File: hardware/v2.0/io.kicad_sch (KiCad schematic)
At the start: 1 part, among them U1 ECP5U-25F-CABGA256

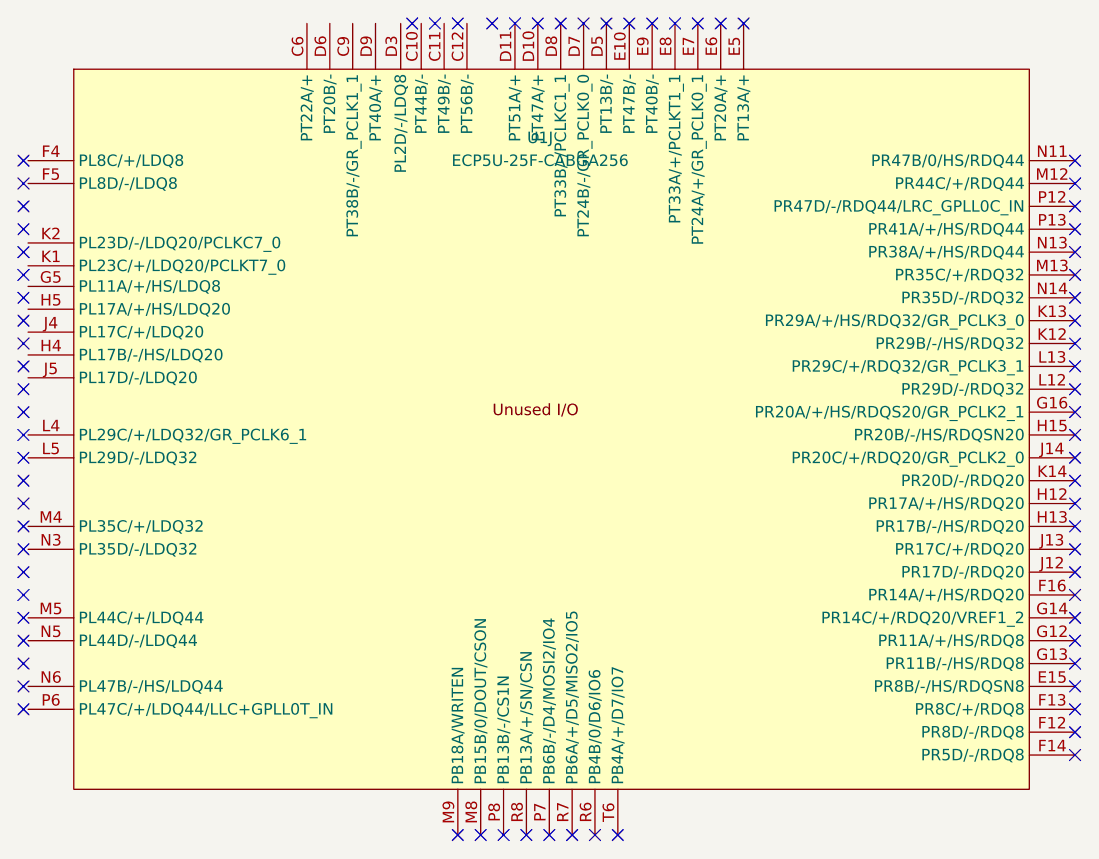
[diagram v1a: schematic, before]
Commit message: ADC SPI SDO
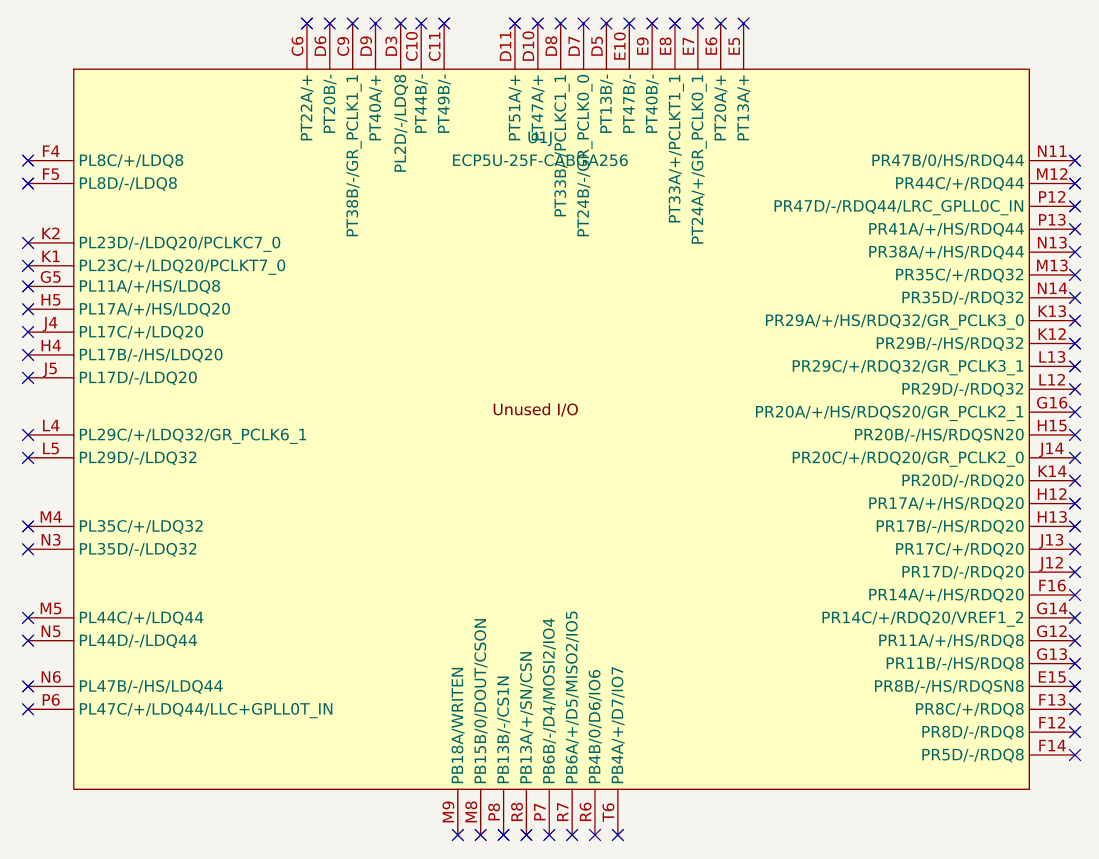
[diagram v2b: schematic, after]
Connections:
- no-connect marks 75 -> 70
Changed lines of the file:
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@@
-	)
-	(no_connect
-		(at 140.97 50.8)
 	)
 	(no_connect
@@
 	)
 	(no_connect
-		(at 97.79 68.58)
-	)
-	(no_connect
 		(at 154.94 50.8)
 	)
@@
 	)
 	(no_connect
-		(at 97.79 71.12)
-	)
-	(no_connect
 		(at 156.21 140.97)
 	)
@@
 	)
 	(no_connect
-		(at 97.79 111.76)
-	)
-	(no_connect
 		(at 214.63 68.58)
 	)
@@
 	)
 	(no_connect
+		(at 136.906 50.8)
+	)
+	(no_connect
+		(at 98.298 75.184)
+	)
+	(no_connect
 		(at 214.63 83.82)
 	)
@@
 	)
 	(no_connect
-		(at 97.79 93.98)
-	)
-	(no_connect
-		(at 97.79 109.22)
+		(at 134.366 50.8)
+	)
+	(no_connect
+		(at 98.298 85.09)
 	)
 	(no_connect
@@
 	)
 	(no_connect
-		(at 97.79 124.46)
-	)
-	(no_connect
-		(at 97.79 99.06)
-	)
-	(no_connect
-		(at 97.79 78.74)
-	)
-	(no_connect
 		(at 214.63 129.54)
 	)
 	(no_connect
-		(at 146.05 50.8)
-	)
-	(no_connect
 		(at 148.59 140.97)
 	)
 	(no_connect
+		(at 98.298 96.52)
+	)
+	(no_connect
 		(at 214.63 101.6)
 	)
@@
 	)
 	(no_connect
+		(at 139.7 50.8)
+	)
+	(no_connect
 		(at 214.63 111.76)
 	)
 	(no_connect
-		(at 149.86 50.8)
-	)
-	(no_connect
-		(at 97.79 116.84)
-	)
-	(no_connect
 		(at 214.63 124.46)
 	)
@@
 	)
 	(no_connect
-		(at 97.79 76.2)
-	)
-	(no_connect
-		(at 97.79 91.44)
-	)
-	(no_connect
-		(at 97.79 83.82)
+		(at 98.298 99.06)
+	)
+	(no_connect
+		(at 98.298 106.68)
 	)
 	(no_connect
@@
 	)
 	(no_connect
-		(at 97.79 88.9)
-	)
-	(no_connect
-		(at 97.79 121.92)
-	)
-	(no_connect
-		(at 97.79 86.36)
-	)
-	(no_connect
-		(at 143.51 50.8)
-	)
-	(no_connect
 		(at 214.63 99.06)
 	)
 	(no_connect
-		(at 97.79 66.04)
+		(at 98.298 119.38)
+	)
+	(no_connect
+		(at 98.298 127)
+	)
+	(no_connect
+		(at 129.286 50.8)
 	)
 	(no_connect
@@
 	)
 	(no_connect
-		(at 97.79 73.66)
-	)
-	(no_connect
 		(at 158.75 140.97)
 	)
 	(no_connect
-		(at 97.79 81.28)
-	)
-	(no_connect
 		(at 151.13 140.97)
 	)
@@
 	)
 	(no_connect
-		(at 97.79 127)
-	)
-	(no_connect
 		(at 214.63 71.12)
 	)
 	(no_connect
-		(at 97.79 114.3)
-	)
-	(no_connect
 		(at 214.63 132.08)
 	)
@@
 	)
 	(no_connect
+		(at 144.526 50.8)
+	)
+	(no_connect
+		(at 98.298 82.55)
+	)
+	(no_connect
 		(at 161.29 140.97)
 	)
@@
 	)
 	(no_connect
-		(at 97.79 106.68)
+		(at 98.298 124.46)
+	)
+	(no_connect
+		(at 98.298 109.22)
+	)
+	(no_connect
+		(at 98.298 90.17)
+	)
+	(no_connect
+		(at 98.298 116.84)
+	)
+	(no_connect
+		(at 98.298 68.58)
 	)
 	(no_connect
@@
 	)
 	(no_connect
+		(at 98.298 77.724)
+	)
+	(no_connect
+		(at 98.298 87.63)
+	)
+	(no_connect
 		(at 214.63 109.22)
 	)
 	(no_connect
+		(at 131.826 50.8)
+	)
+	(no_connect
 		(at 214.63 119.38)
 	)
 	(no_connect
+		(at 141.986 50.8)
+	)
+	(no_connect
 		(at 214.63 73.66)
 	)
 	(no_connect
-		(at 97.79 101.6)
-	)
-	(no_connect
-		(at 97.79 119.38)
+		(at 98.298 66.04)
 	)
 	(no_connect
@@
 	)
 	(no_connect
-		(at 97.79 104.14)
+		(at 98.298 80.01)
 	)
 	(no_connect
@@
 	)
 	(no_connect
-		(at 97.79 96.52)
-	)
-	(no_connect
